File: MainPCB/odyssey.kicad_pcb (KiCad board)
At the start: 2 copper layers, 26.2 x 24 mm, 8 parts, among them J1 MSD-4-A, U1 I3G4250DTR, U2 IIS2MDCTR, U3 XIAO-RP2040-SMD, U4 TL3305AF260QG, U5 MPL3115A2

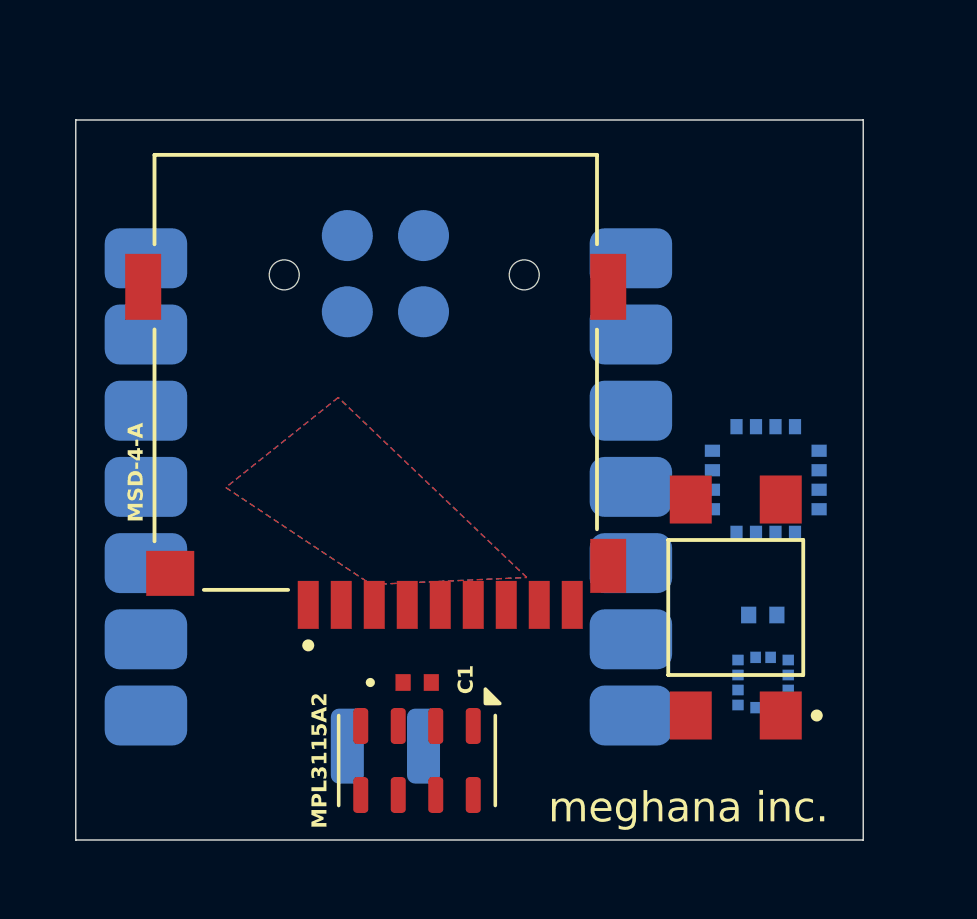
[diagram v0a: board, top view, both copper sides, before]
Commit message: updating main pcb
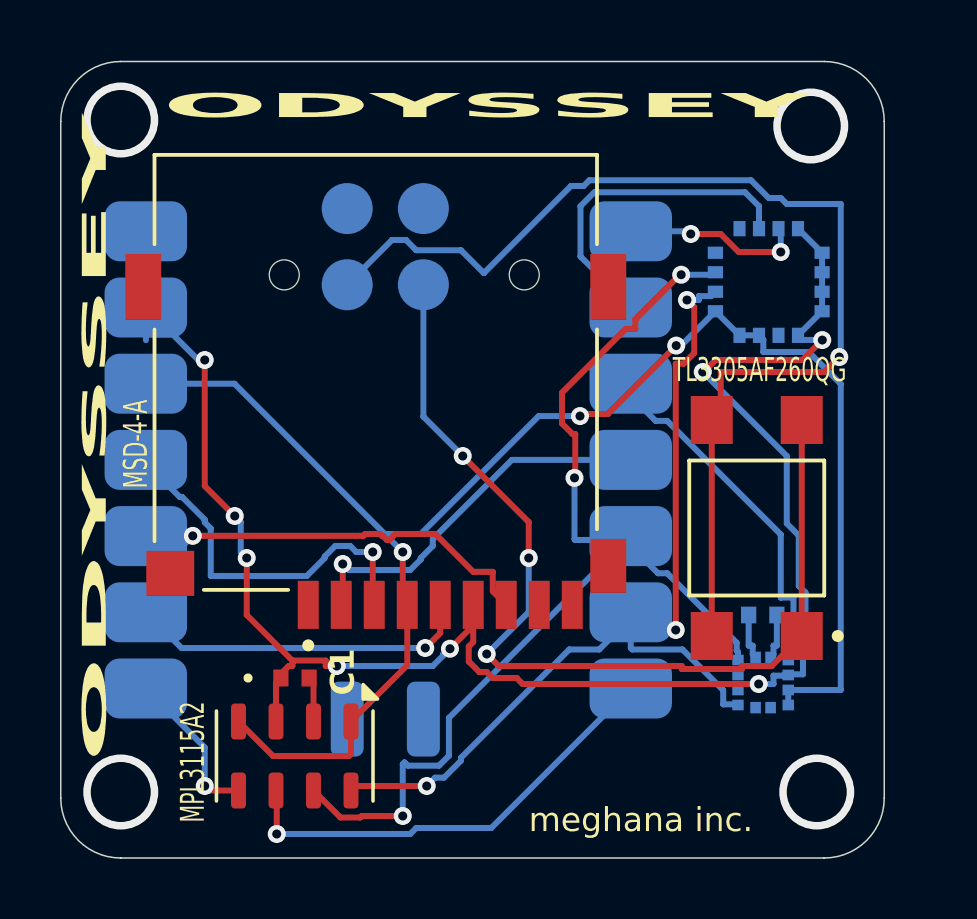
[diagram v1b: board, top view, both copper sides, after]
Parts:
- C1: value C1 -> 0402B104K160CT
- moved U1 6.60 mm to (77.6, 50.4)
- moved C1 4.08 mm to (61.8, 63.6)
- moved U5 4.08 mm to (61.8, 66.2)
- moved U4 2.74 mm to (77.2, 58.6)
- moved U3 0.90 mm to (65.0, 56.3)
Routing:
- net GND: track 1.00 -> 60.1 mm, vias 0 -> 8
- net 3.3V XIAO: track 0.00 -> 54.7 mm, vias 0 -> 3
- net Net-(U3-GND-Pad20): track 0.00 -> 37.3 mm, vias 0 -> 1
- net XIAO SDA: track 0.00 -> 36.5 mm, vias 0 -> 3
- net Net-(U3-RST): track 0.00 -> 33.0 mm, vias 0 -> 3
- net XIAO SCL: track 0.00 -> 32.2 mm, vias 0 -> 3
- net MPL INT1: track 0.00 -> 15.3 mm, vias 0 -> 1
- net MISO: track 0.00 -> 14.0 mm, vias 0 -> 1
- net MSD STAT: track 0.00 -> 12.8 mm, vias 0 -> 1
- net MOSI: track 0.00 -> 12.5 mm, vias 0 -> 1
- net IIS2 INT: track 0.00 -> 12.2 mm
- net CLK: track 0.00 -> 11.5 mm, vias 0 -> 1
- net I3G4 INT2: track 0.00 -> 11.2 mm
- net I3G4 INT1: track 0.00 -> 6.09 mm, vias 0 -> 2
- net MPL INT2: track 0.00 -> 5.25 mm, vias 0 -> 1
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- removed copper zone on B.Cu, net GND
- removed copper zone on F.Cu, net GND
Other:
- board size 26.2 x 24 mm -> 27.5 x 26.5 mm
- board text added: "C1"
- board text added: "ODYSSEY"
- board text added: "TL3305AF260QG"
